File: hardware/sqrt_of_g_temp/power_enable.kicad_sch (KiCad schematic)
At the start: 7 parts, among them Q5 NDS8434

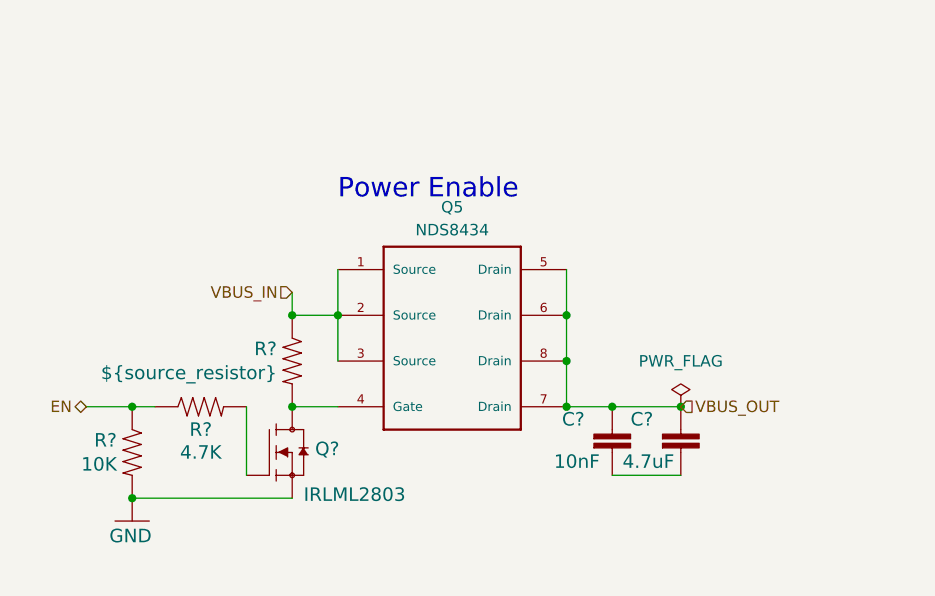
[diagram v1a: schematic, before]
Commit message: ads board 1.0.1
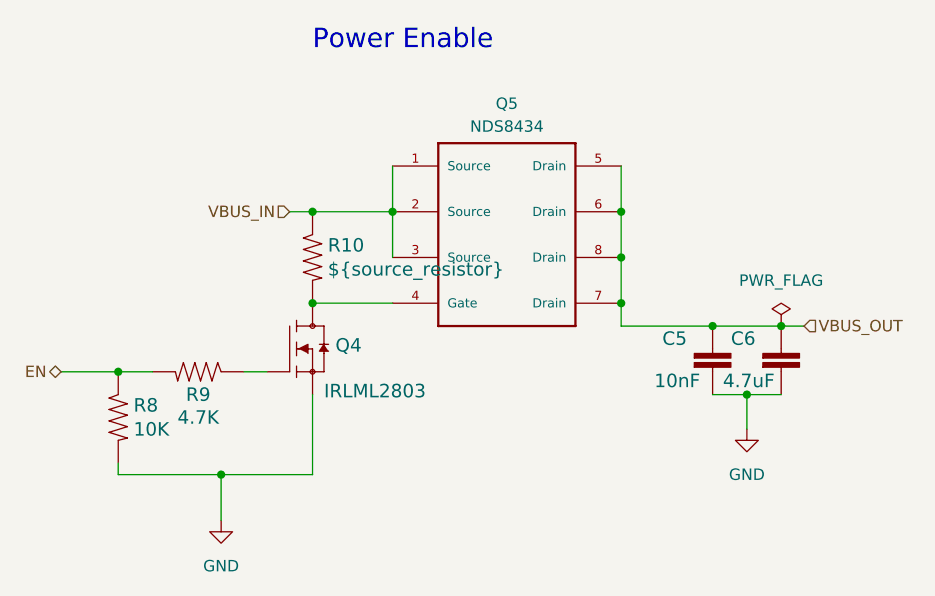
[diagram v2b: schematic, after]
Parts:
- removed Q?: IRLML2803, mainboard:SOT-23, symbol mainboard:IRLML2803TRPBF
- added Q4: IRLML2803, mainboard:SOT-23, symbol mainboard:IRLML2803TRPBF
- C5, C6: renamed from C?; footprint Capacitor_SMD:C_0603_1608Metric -> Capacitor_SMD:C_0402_1005Metric
- R10, R8, R9: renamed from R?; footprint Resistor_SMD:R_0603_1608Metric -> Resistor_SMD:R_0402_1005Metric
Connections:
- net EN: now also R9.2; no longer R9.1
- net GND: now also C5.2, C6.2, Q4.2 (S)
- net at Q5.4 (Gate), R10.2: now also Q4.3 (D)
- new net: Q4.1 (G), R9.1
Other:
- title: (none) -> √g
- moved on the sheet: C5, C6, R10, R8, R9
